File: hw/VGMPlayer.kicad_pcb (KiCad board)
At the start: 4 copper layers, 40 x 67 mm, 99 parts, among them J1 Micro_SD_Card, J2 EarPiece, P1 USB_C_Receptacle_16P, P2 SWD, P3 BATT, P5 ICSP, P6 CODEC, Q1 AO3401A, Q2 AO3401A, Q3 2N7002, Q4 2N7002, U1 RP2040, U2 W25QxxJVZP, U3 LP5907MFX-3.3, U4 WM8978, U5 MCP73831-OT, U6 PIC16F1503-IMG, U7 LP5907MFX-3.3, Y1 12MHz

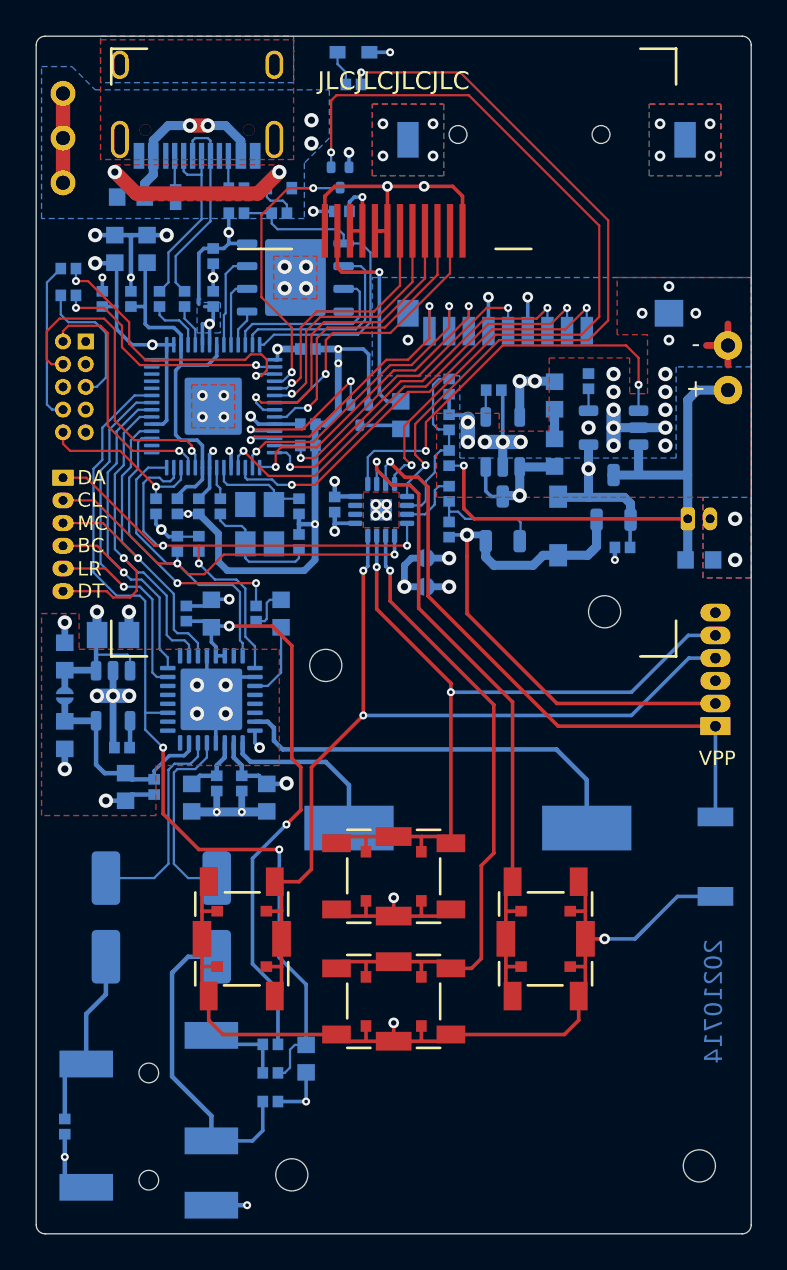
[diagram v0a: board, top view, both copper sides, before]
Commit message: V4 hardware
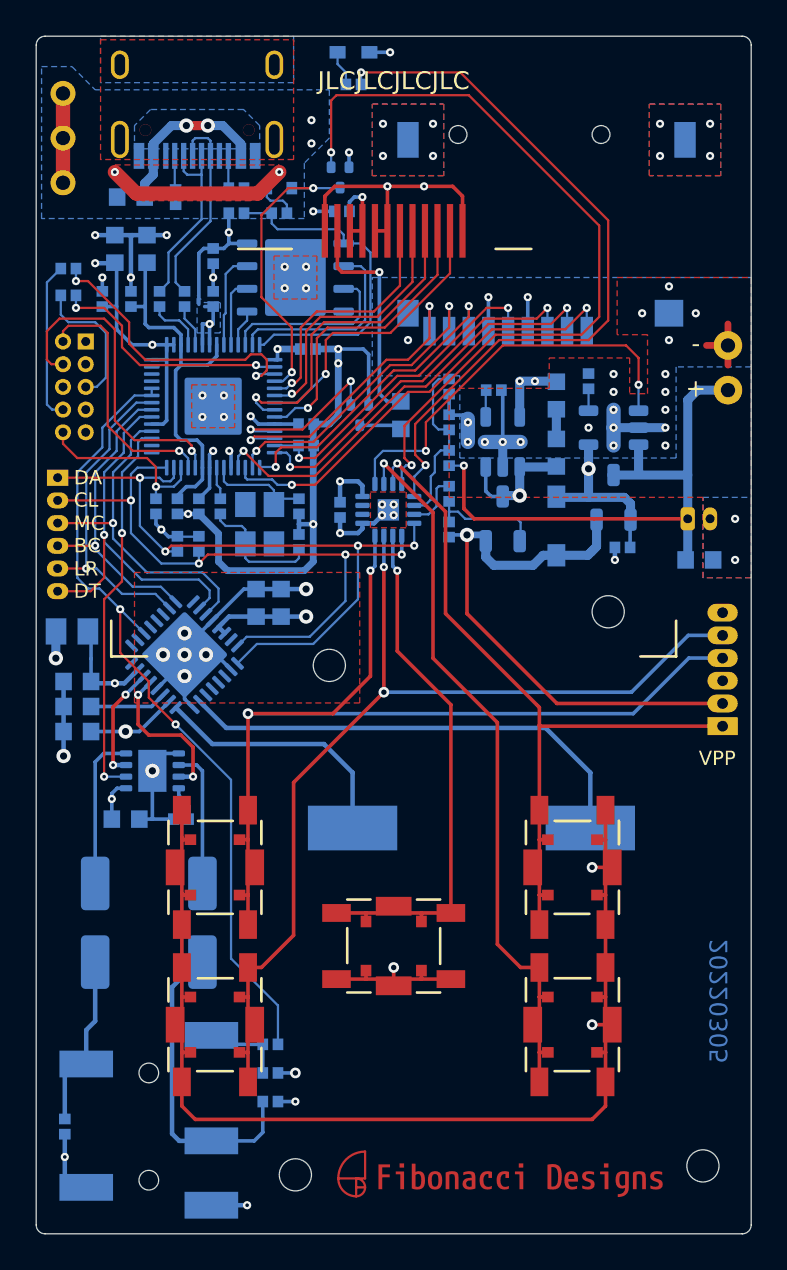
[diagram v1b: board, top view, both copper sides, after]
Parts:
- removed C14: 1u, BZ_Capacitor:C_0603
- removed the C17 at (138.4, 109.3)
- removed the C19 at (136.6, 119.0)
- removed the C23 at (131.6, 111.7)
- removed the C24 at (134.8, 116.8)
- removed the C27 at (140.1, 118.8)
- removed the C30 at (145.1, 134.2)
- removed JP1: Jumper-NC, BZ_Misc:Jumper-Solder
- removed JP2, JP3: Jumper-NO, BZ_Misc:Jumper-Solder
- removed R13: 1K, BZ_Resistor:R_0402
- removed the U3 at (134.3, 113.9)
- added C20: 1u, BZ_Capacitor:C_0603, B.Cu at (135.0, 120.8)
- added U4: MAX9890BETA, BZ_Standard_IC:TDFN-8-1EP_3x3x0.65P_EP2.3x1.5, B.Cu at (136.5, 118.1)
- added kibuzzard-62236962: G***, kibuzzard-62236962, F.Cu at (157.1, 141.0)
- C15: renamed from C25; value 10u -> 4.7u
- C16: renamed from C18; value 10u -> 4.7u
- C17: renamed from C20; value 10u -> 4.7u
- C18: renamed from C22; value 10u -> 4.7u
- C19: renamed from C26; value 10u -> 4.7u
- S1: value M -> B
- S2: value P -> F
- S5: value RESET -> P; footprint BZ_Switch:SW-PUSH_4x3x2H -> VGMPlayer:MultiButton; moved to F.Cu
- moved C15 13.0 mm to (142.3, 108.7), turned to 90 degrees
- moved S3 13.0 mm to (140.0, 132.3), turned to 90 degrees
- moved C18 11.2 mm to (132.3, 115.9), turned to 180 degrees
- moved C19 8.18 mm to (132.3, 114.5), turned to 180 degrees
- moved S5 8.02 mm to (160.0, 123.5), turned to -90 degrees
- moved C17 6.49 mm to (132.3, 113.1), turned to 180 degrees
- moved S2 5.03 mm to (160.0, 132.3)
- moved S1 4.27 mm to (140.0, 123.5)
- moved C16 3.95 mm to (143.7, 108.7)
- moved C21 3.94 mm to (138.1, 120.8), turned to 180 degrees
- moved S4 3.10 mm to (150.0, 127.9)
- moved U3 2.92 mm to (138.3, 111.6), turned to 45 degrees
- moved FB1 2.31 mm to (132.0, 110.3), turned to 180 degrees
- moved R15 1.60 mm to (143.1, 133.4)
- moved R17 1.60 mm to (143.1, 135.0)
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- renumbered C28 to C22, C29 to C23, C16 to C24, C31 to C25, C33 to C26, C34 to C27, C35 to C28, C32 to C29, C36 to C30, U4 to U3
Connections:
- C15 pad 1: VDDA -> 3V3
- C17 pad 1: VDDA -> /AVDD
- C18 pad 1: Net-(C21-Pad1) -> VIN
- C22 pad 1: Net-(C28-Pad1) -> Net-(C22-Pad1)
- C23 pad 1: Net-(C29-Pad1) -> Net-(C23-Pad1)
- C26 pad 1: Net-(C33-Pad1) -> VIN
- FB1 pad 1: Net-(C21-Pad1) -> /AVDD
- FB1 pad 2: VIN -> 3V3
- P1 pad A8: (no net) -> unconnected-(P1-PadA8)
- P1 pad B8: (no net) -> unconnected-(P1-PadB8)
- P2 pad 6: (no net) -> unconnected-(P2-Pad6)
- P2 pad 7: (no net) -> unconnected-(P2-Pad7)
- P5 pad 6: (no net) -> unconnected-(P5-Pad6)
- Q2 pad 3: Net-(C33-Pad1) -> VIN
- U1 pad 29: (no net) -> unconnected-(U1-Pad29)
- U1 pad 30: (no net) -> unconnected-(U1-Pad30)
- U1 pad 31: Net-(R13-Pad2) -> /OUTEN
- U1 pad 38: (no net) -> /JACK_DET
- U1 pad 39: (no net) -> unconnected-(U1-Pad39)
- U1 pad 40: (no net) -> unconnected-(U1-Pad40)
- U1 pad 41: (no net) -> unconnected-(U1-Pad41)
- U3 pad 1: (no net) -> unconnected-(U3-Pad1)
- U3 pad 15: (no net) -> unconnected-(U3-Pad15)
- U3 pad 19: /BEEP -> unconnected-(U3-Pad19)
- U3 pad 2: (no net) -> unconnected-(U3-Pad2)
- U3 pad 20: (no net) -> unconnected-(U3-Pad20)
- U3 pad 21: (no net) -> unconnected-(U3-Pad21)
- U3 pad 22: (no net) -> unconnected-(U3-Pad22)
- U3 pad 26: Net-(C21-Pad1) -> VIN
- U3 pad 29: Net-(C28-Pad1) -> Net-(U3-Pad29)
- U3 pad 30: Net-(C29-Pad1) -> Net-(U3-Pad30)
- U3 pad 31: VDDA -> /AVDD
- U3 pad 32: (no net) -> unconnected-(U3-Pad32)
- U3 pad 4: (no net) -> unconnected-(U3-Pad4)
- U3 pad 5: (no net) -> unconnected-(U3-Pad5)
- U3 pad 6: (no net) -> unconnected-(U3-Pad6)
- U3 pad 9: (no net) -> unconnected-(U3-Pad9)
- U7 pad 1: Net-(C33-Pad1) -> VIN
- U7 pad 3: Net-(C33-Pad1) -> VIN
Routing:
- net 3V3: track 109.5 -> 156.2 mm
- net Net-(C21-Pad1): track 31.0 -> 1.95 mm, vias 2 -> 0
- net VIN: track 23.6 -> 45.6 mm
- net /OUTEN: track 0.00 -> 21.4 mm, vias 0 -> 2
- net /AVDD: track 0.00 -> 16.9 mm, vias 0 -> 2
- net Net-(R13-Pad2): track 15.8 -> 0.00 mm, vias 2 -> 0
- net Net-(C33-Pad1): track 14.7 -> 0.00 mm, vias 2 -> 0
- net VDDA: track 12.2 -> 0.00 mm
- net /ICSPCLK: track 43.5 -> 55.7 mm
- net Net-(C29-Pad1): track 11.8 -> 0.00 mm
- net Net-(C28-Pad1): track 10.8 -> 0.00 mm
- net Net-(U3-Pad29): track 0.00 -> 8.80 mm, vias 0 -> 2
- net Net-(C23-Pad1): track 0.00 -> 8.52 mm
- net Net-(C22-Pad1): track 0.00 -> 7.86 mm
- net /VPP: track 34.4 -> 41.9 mm
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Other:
- rule solder_mask_min_width: 0.08 -> 0.2
- board text added: "20220305"
- board text removed: "20210714"

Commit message: V4 hardware send for JLC
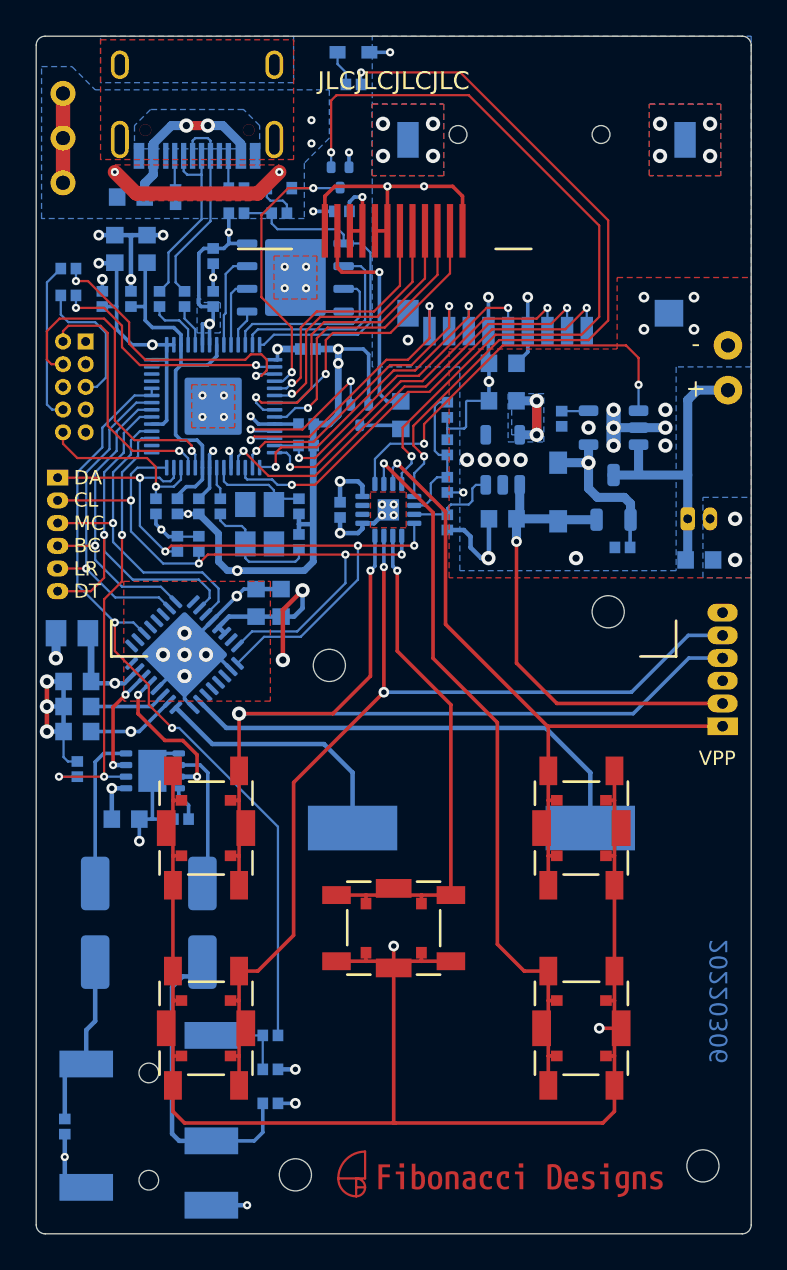
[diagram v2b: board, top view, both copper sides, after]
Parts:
- removed the C27 at (155.6, 96.8)
- removed Q2: AO3401A, BZ_Standard_IC:SOT-23-3
- removed R20: 100K, BZ_Resistor:R_0402
- added C29: 4.7u, BZ_Capacitor:C_0603, B.Cu at (156.1, 95.3)
- added R13: 10K, BZ_Resistor:R_0402, B.Cu at (132.3, 118.0)
- C26: value 1u -> 4.7u
- R21: value 10K -> 100K
- S1: value B -> U
- S2: value F -> B
- S3: value U -> D
- S4: value D -> P
- S5: value P -> F
- U7: value LP5907MFX-3.3 -> XC6220B331MR
- moved C25 7.52 mm to (156.1, 104.0), turned to 180 degrees
- moved C26 4.17 mm to (156.1, 97.4), turned to 180 degrees
- moved R18 2.58 mm to (159.4, 98.4), turned to -90 degrees
- moved S1 2.26 mm to (139.5, 121.3)
- moved S5 2.26 mm to (160.5, 121.3)
- moved D2 1.90 mm to (159.2, 102.5)
- moved R21 1.60 mm to (153.0, 104.2), turned to -90 degrees
- moved R23 1.50 mm to (153.0, 102.1)
- moved R24 1.40 mm to (153.0, 100.0)
- moved C28 1.30 mm to (153.0, 97.9)
- moved S4 1.00 mm to (150.0, 126.9)
- moved U7 1.00 mm to (156.1, 100.7)
- moved S2 0.54 mm to (160.5, 132.5)
- moved S3 0.54 mm to (139.5, 132.5)
- moved R15 0.50 mm to (143.1, 132.9)
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- renumbered C15 to C14, C16 to C15, C17 to C16, C18 to C17, C20 to C18, C21 to C19, C19 to C20, C22 to C21, C23 to C22, C24 to C23, C25 to C24, C28 to C25, C29 to C27, C30 to C28
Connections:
- C17 pad 1: VIN -> /AVDD
- C25 pad 1: 3V3 -> VRAW
- C26 pad 1: VIN -> 3V3
- R21 pad 1: Net-(Q2-Pad1) -> Net-(R21-Pad1)
- R21 pad 2: Net-(R21-Pad2) -> GND
- U3 pad 26: VIN -> /AVDD
- U6 pad 7: Net-(R21-Pad2) -> Net-(R21-Pad1)
- U7 pad 1: VIN -> VRAW
- U7 pad 3: VIN -> Net-(R21-Pad1)
- U7 pad 4: Net-(C27-Pad1) -> unconnected-(U7-Pad4)
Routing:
- net VIN: track 45.6 -> 0.00 mm, vias 2 -> 0
- net 3V3: track 156.2 -> 141.1 mm, vias 15 -> 16
- net GND: track 219.3 -> 230.7 mm, vias 79 -> 77
- net Net-(Q2-Pad1): track 6.19 -> 0.00 mm
- net Net-(R21-Pad1): track 0.00 -> 5.33 mm
- net VRAW: track 45.3 -> 41.5 mm
- net /OUTEN: track 21.4 -> 25.0 mm, vias 2 -> 3
- net Net-(R21-Pad2): track 3.19 -> 0.00 mm
- net /AVDD: track 16.9 -> 20.0 mm, vias 2 -> 3
- net /VPP: track 41.9 -> 39.4 mm
- net /BATT: track 33.3 -> 31.4 mm
- net Net-(C28-Pad1): track 10.1 -> 8.37 mm
- net Net-(C27-Pad1): track 1.35 -> 0.00 mm
- net /ICSPDAT: track 56.6 -> 55.4 mm
- net Net-(S4-Pad2): track 30.1 -> 29.1 mm
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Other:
- rule pad_to_mask_clearance: 0.05 -> 0
- board text added: "20220306"
- board text removed: "20220305"
